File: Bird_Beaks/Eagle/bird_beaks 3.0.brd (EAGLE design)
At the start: 172.7 x 106.4 mm, 29 parts, among them U1 ADAFRUIT_ITSYBITSY_5V, X1 PHOENIX_508_3PIN, X10 PHOENIX_508_3PIN, X11 PHOENIX_508_4PIN, X2 PHOENIX_508_3PIN, X3 PHOENIX_508_3PIN, X4 PHOENIX_508_2PIN, X5 PHOENIX_508_4PIN, X6 PHOENIX_508_4PIN, X7 PHOENIX_508_3PIN, X8 PHOENIX_508_3PIN, X9 PHOENIX_508_3PIN

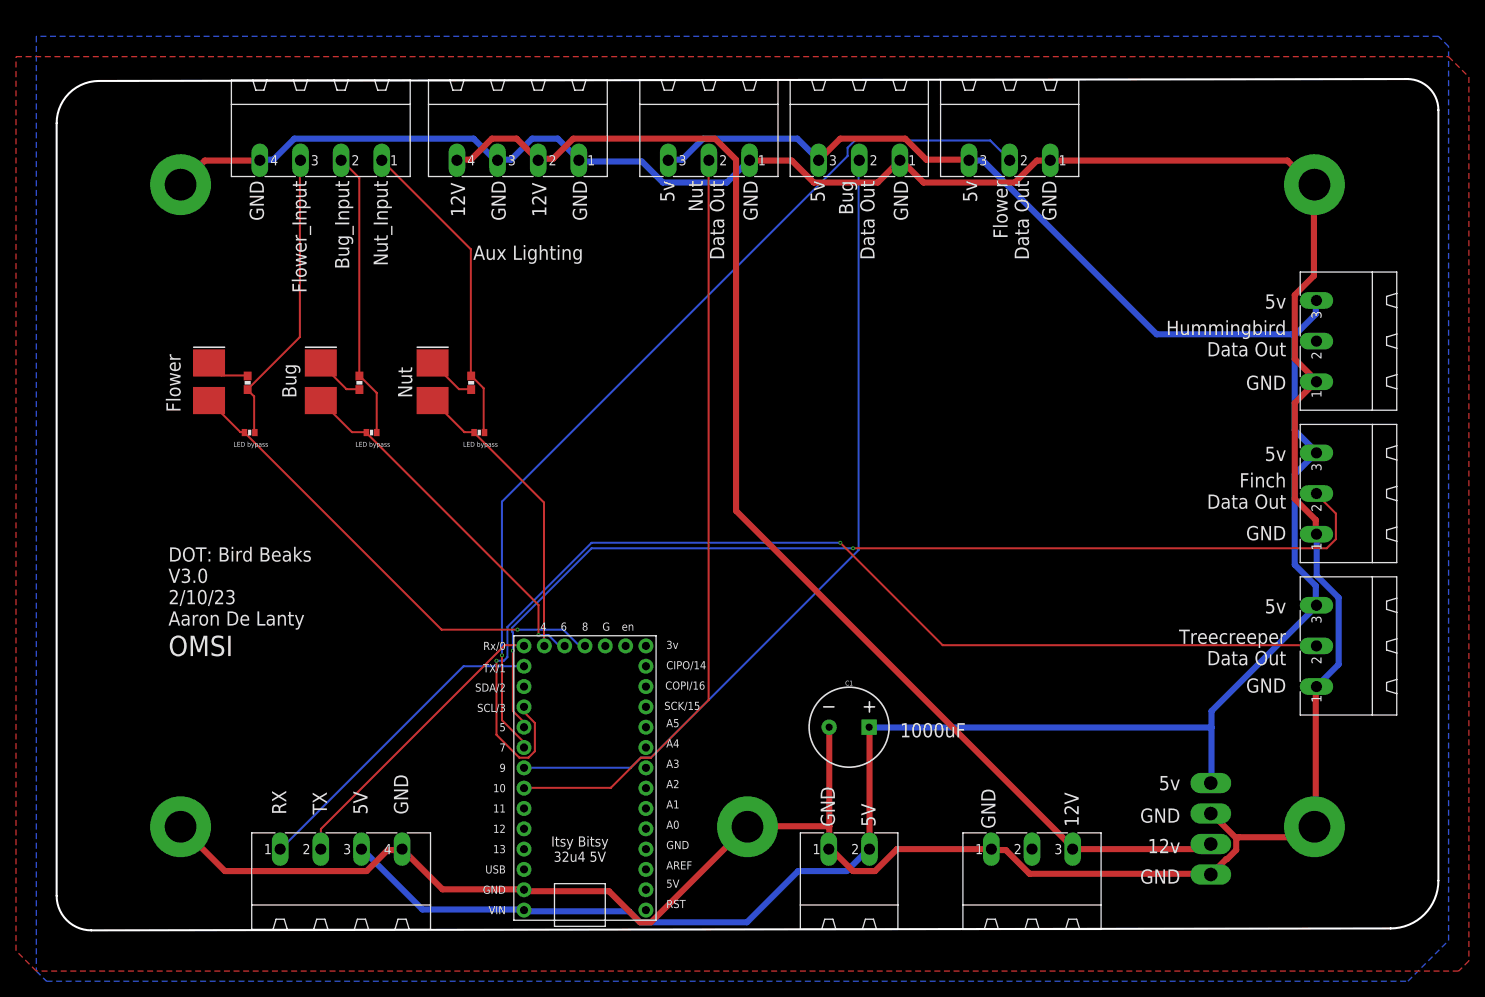
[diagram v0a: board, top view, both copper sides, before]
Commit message: Revision for output
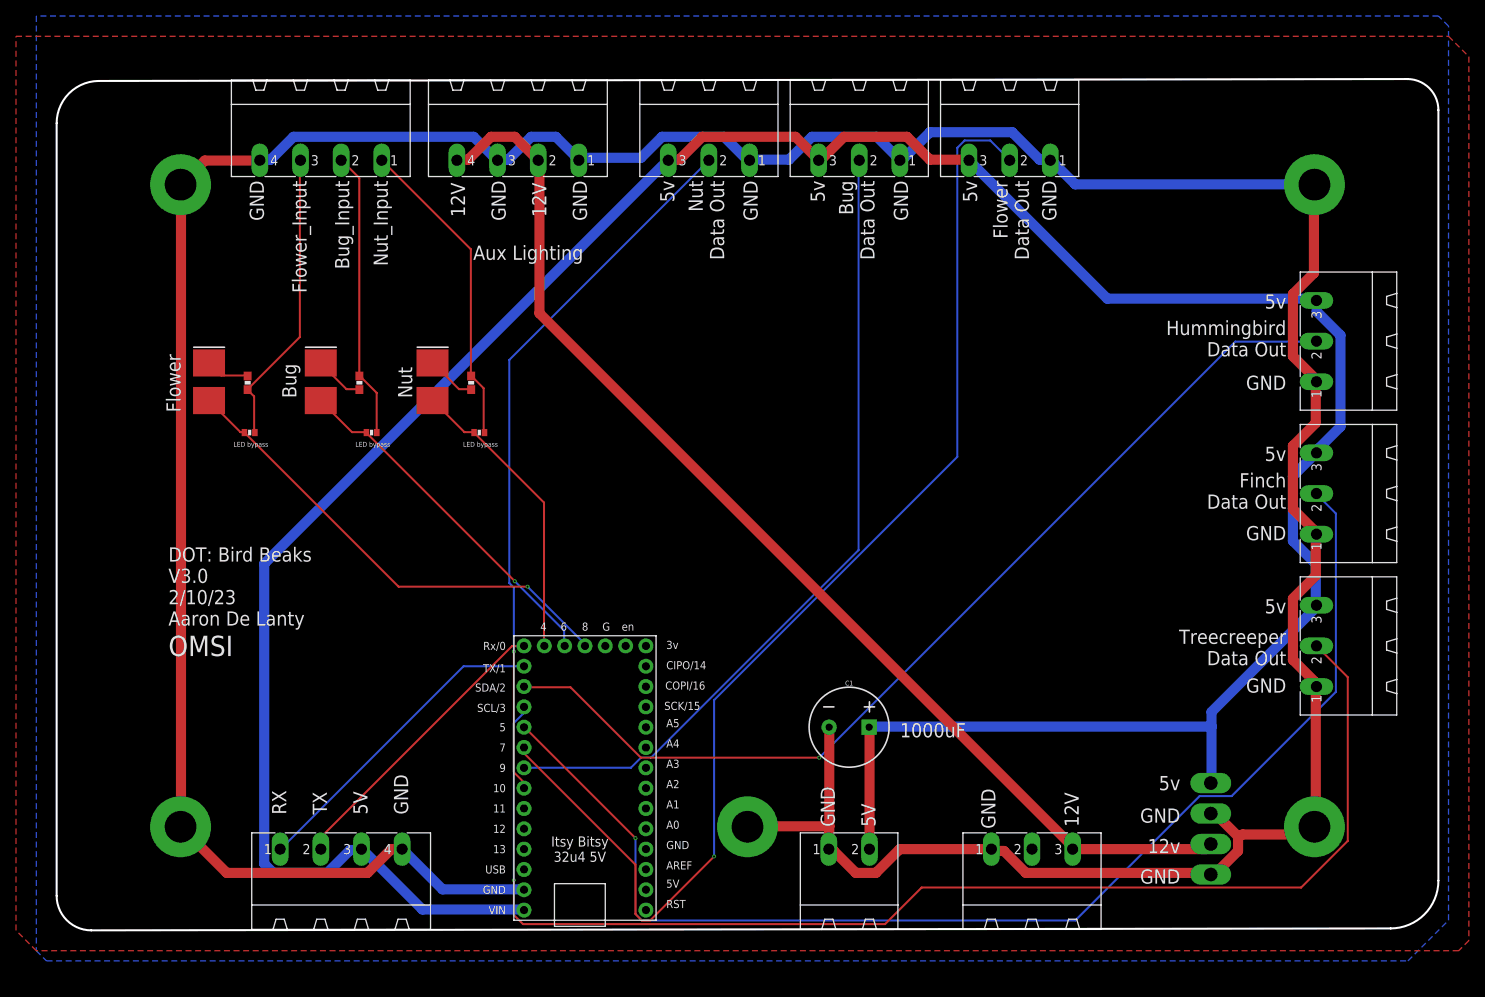
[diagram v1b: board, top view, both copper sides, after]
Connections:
- removed net HUMMINGIRD_OUTPUT: U1.SDA
- net HUMMINGBIRD_OUTPUT: now also U1.SDA
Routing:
- net HUMMINGBIRD_OUTPUT: track 0.00 -> 124.3 mm, vias 0 -> 1
- net 5V: track 291.4 -> 368.1 mm
- net GND: track 423.1 -> 471.1 mm
- net FLOWER_OUTPUT: track 115.7 -> 149.3 mm
- net FINCH_OUTPUT: track 127.3 -> 154.7 mm, vias 2 -> 1
- net TREECREEPER_OUTPUT: track 137.9 -> 161.5 mm, vias 2 -> 1
- net 12V: track 160.5 -> 143.8 mm
- net NUT_OUTPUT: track 95.1 -> 89.6 mm, vias 0 -> 1
- net N$5: track 45.4 -> 44.3 mm
- net N$10: track 37.5 -> 36.8 mm
